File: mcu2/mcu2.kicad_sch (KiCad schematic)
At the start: 30 parts, among them J1 KF128-5.08, J2 Conn_01x26, J3 Conn_01x02, J4 Conn_01x01, J5 Conn_01x01, J6 Conn_01x01, J7 Conn_01x02, J8 Conn_01x26, Q1 WSF3085, Q2 PL4009, Q3 PL4009, U1 rp2040_zero, U2 motor_driver

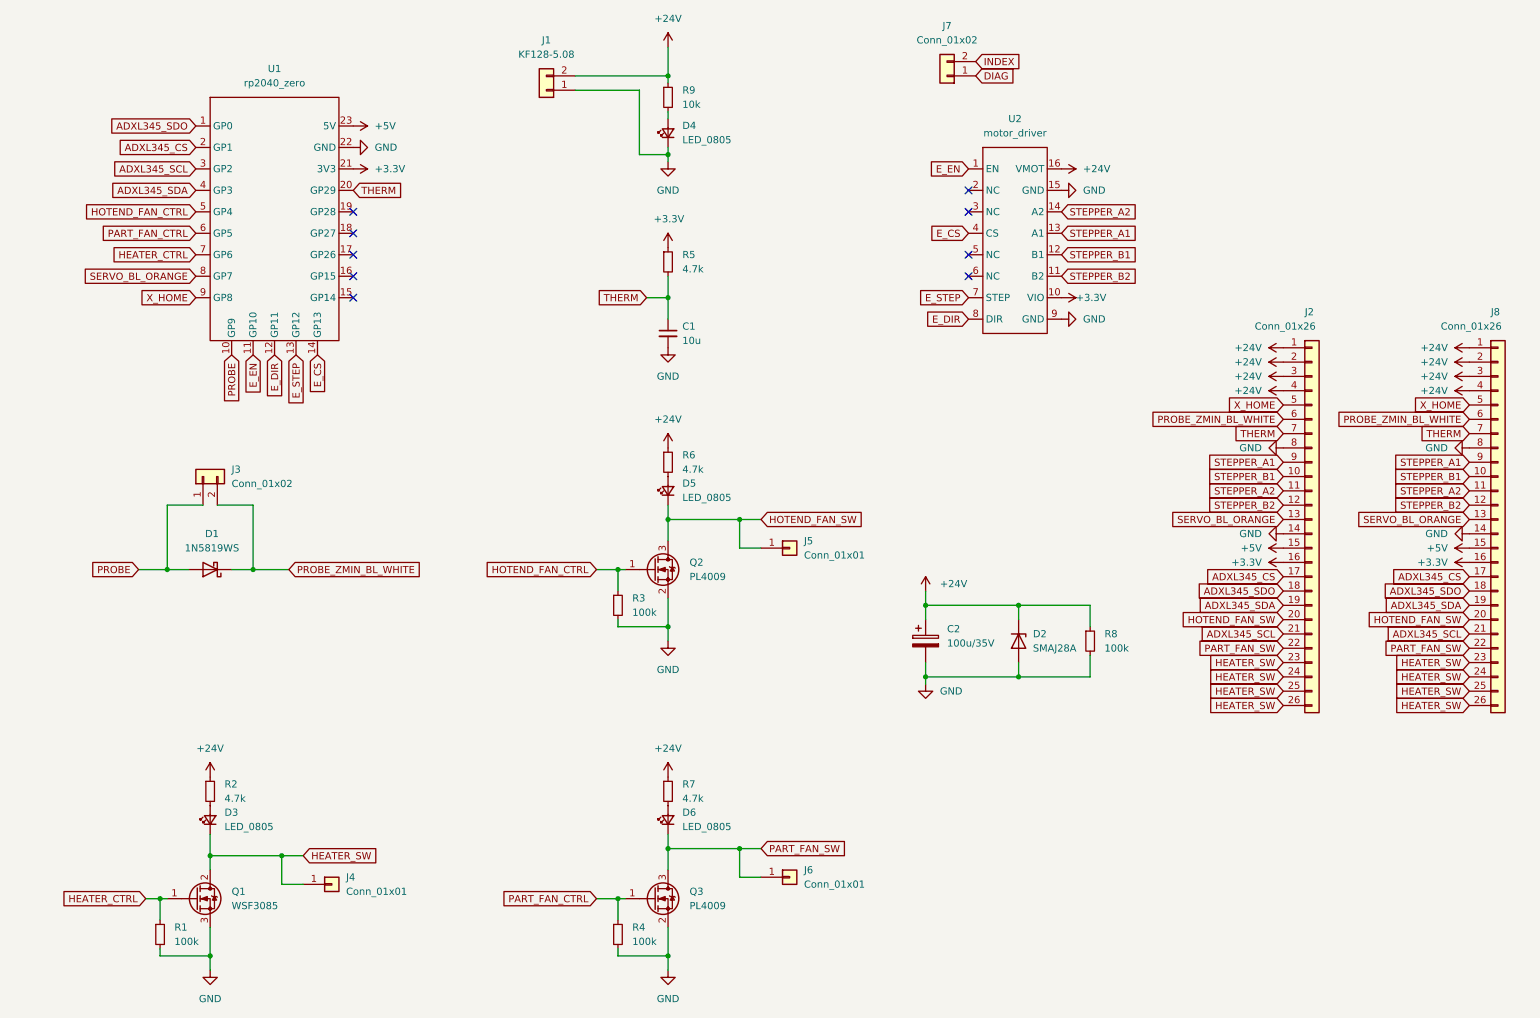
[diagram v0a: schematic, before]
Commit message: mcu schematic r3
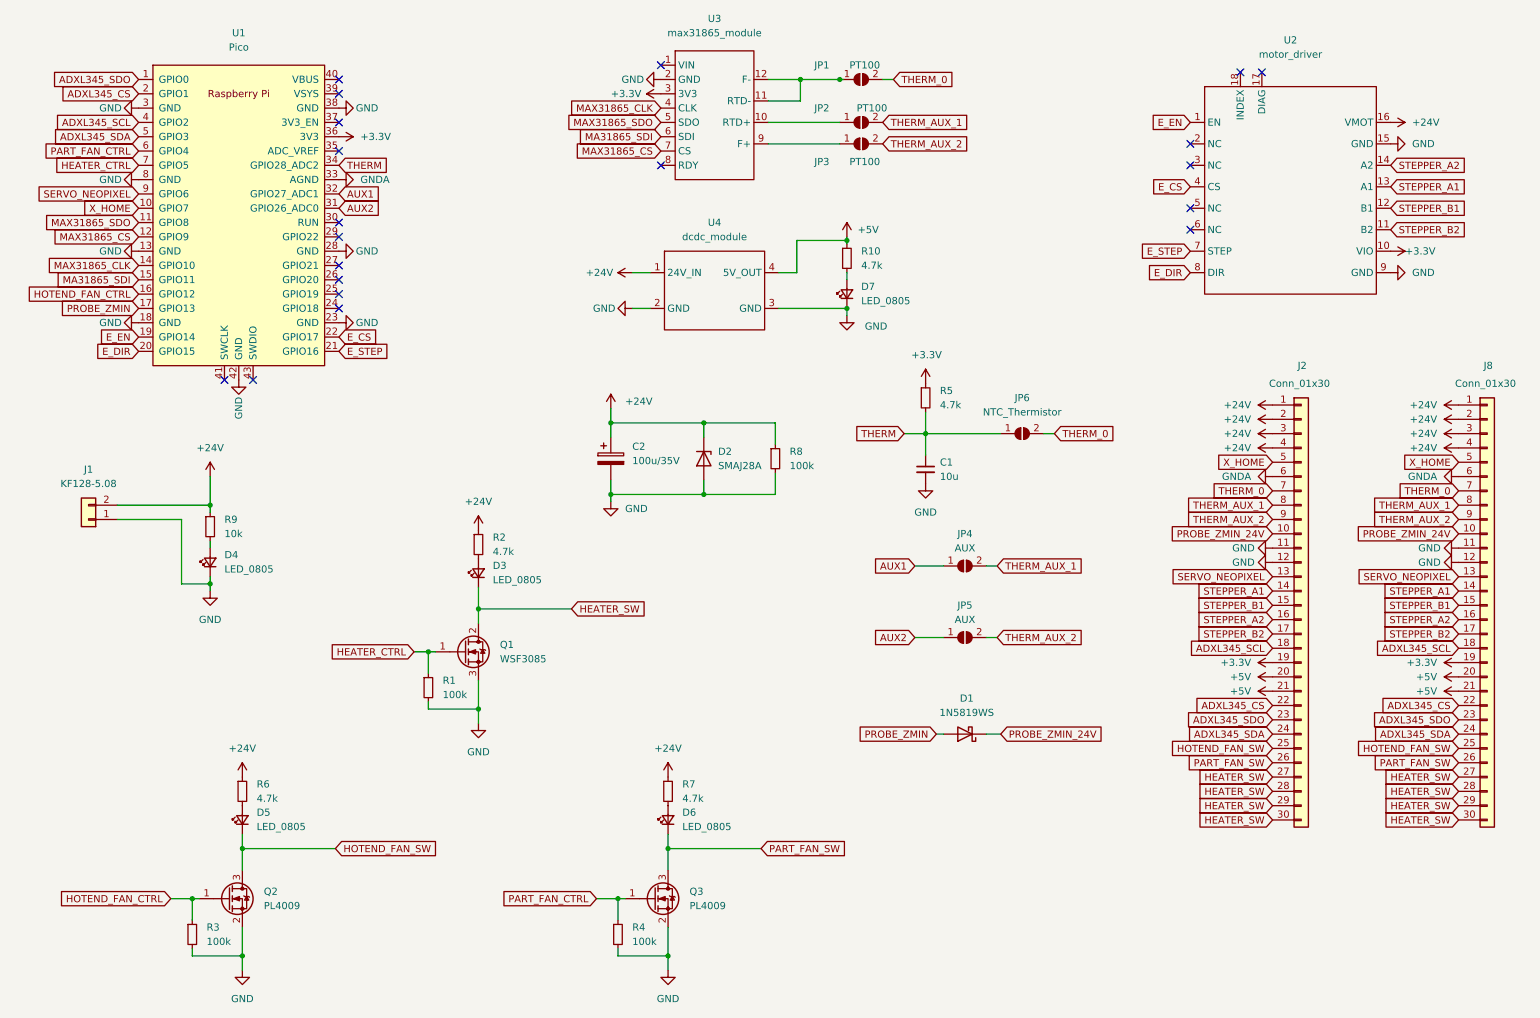
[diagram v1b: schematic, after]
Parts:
- removed J2, J8: Conn_01x26, FFCconnector:FFC26pinTH, symbol Connector_Generic:Conn_01x26
- removed J3, J7: Conn_01x02, Connector_PinHeader_2.54mm:PinHeader_1x02_P2.54mm_Vertical, symbol Connector_Generic:Conn_01x02
- removed J4, J5, J6: Conn_01x01, Connector_PinHeader_2.54mm:PinHeader_1x01_P2.54mm_Vertical, symbol Connector_Generic:Conn_01x01
- removed U1: rp2040_zero, rp2040_zero:RP2040Zero, symbol rp2040_zero:rp2040_zero
- removed U2: motor_driver, motor_driver:DIP-16_500, symbol motor_driver:motor_driver
- added D7: LED_0805, LED_SMD:LED_0805_2012Metric_Pad1.15x1.40mm_HandSolder, symbol Device:LED_Small
- added J2, J8: Conn_01x30, ffc_connectors:ffc-30pin, symbol Connector_Generic:Conn_01x30
- added JP1, JP2, JP3: PT100, symbol Jumper:SolderJumper_2_Open
- added JP4, JP5: AUX, symbol Jumper:SolderJumper_2_Open
- added JP6: NTC_Thermistor, symbol Jumper:SolderJumper_2_Open
- added R10: 4.7k, Resistor_SMD:R_0805_2012Metric_Pad1.20x1.40mm_HandSolder, symbol Device:R_Small
- added U1: Pico, RPi_Pico:RPi_Pico_SMD_TH, symbol RPi_Pico:Pico
- added U2: motor_driver, symbol ffc_mcu_library:motor_driver
- added U3: max31865_module, symbol ffc_mcu_library:max31865_module
- added U4: dcdc_module, symbol ffc_mcu_library:dcdc_module
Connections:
- net +24V: now also J2.1 (Pin_1), J2.2 (Pin_2), J2.3 (Pin_3), J2.4 (Pin_4), J8.1 (Pin_1), J8.2 (Pin_2), J8.3 (Pin_3), J8.4 (Pin_4), U2.16 (VMOT), U4.1 (24V_IN)
- net +3V3: now also J2.19 (Pin_19), J8.19 (Pin_19), U1.36 (3V3), U2.10 (VIO), U3.3 (3V3)
- net +5V: now also J2.20 (Pin_20), J2.21 (Pin_21), J8.20 (Pin_20), J8.21 (Pin_21), R10.1, U4.4 (5V_OUT)
- net ADXL345_CS: now also J2.22 (Pin_22), J8.22 (Pin_22), U1.2 (GPIO1)
- net ADXL345_SCL: now also J2.18 (Pin_18), J8.18 (Pin_18), U1.4 (GPIO2)
- net ADXL345_SDA: now also J2.24 (Pin_24), J8.24 (Pin_24), U1.5 (GPIO3)
- net ADXL345_SDO: now also J2.23 (Pin_23), J8.23 (Pin_23), U1.1 (GPIO0)
- net E_CS: now also U1.22 (GPIO17), U2.4 (CS)
- net E_DIR: now also U1.20 (GPIO15), U2.8 (DIR)
- net E_EN: now also U1.19 (GPIO14), U2.1 (EN)
- net E_STEP: now also U1.21 (GPIO16), U2.7 (STEP)
- net GND: now also D7.1 (K), J2.11 (Pin_11), J2.12 (Pin_12), J8.11 (Pin_11), J8.12 (Pin_12), U1.13 (GND), U1.18 (GND), U1.23 (GND), U1.28 (GND), U1.3 (GND), U1.38 (GND), U1.42 (GND), U1.8 (GND), U2.15 (GND), U2.9 (GND), U3.2 (GND), U4.2 (GND), U4.3 (GND)
- net HEATER_CTRL: now also U1.7 (GPIO5)
- net HEATER_SW: now also J2.27 (Pin_27), J2.28 (Pin_28), J2.29 (Pin_29), J2.30 (Pin_30), J8.27 (Pin_27), J8.28 (Pin_28), J8.29 (Pin_29), J8.30 (Pin_30)
- net HOTEND_FAN_CTRL: now also U1.16 (GPIO12)
- net HOTEND_FAN_SW: now also J2.25 (Pin_25), J8.25 (Pin_25)
- net PART_FAN_CTRL: now also U1.6 (GPIO4)
- net PART_FAN_SW: now also J2.26 (Pin_26), J8.26 (Pin_26)
- net STEPPER_A1: now also J2.14 (Pin_14), J8.14 (Pin_14), U2.13 (A1)
- net STEPPER_A2: now also J2.16 (Pin_16), J8.16 (Pin_16), U2.14 (A2)
- net STEPPER_B1: now also J2.15 (Pin_15), J8.15 (Pin_15), U2.12 (B1)
- net STEPPER_B2: now also J2.17 (Pin_17), J8.17 (Pin_17), U2.11 (B2)
- net THERM: now also JP6.1 (A), U1.34 (GPIO28_ADC2)
- net X_HOME: now also J2.5 (Pin_5), J8.5 (Pin_5), U1.10 (GPIO7)
- net PROBE renamed PROBE_ZMIN
- net PROBE_ZMIN: now also U1.17 (GPIO13)
- net PROBE_ZMIN_BL_WHITE renamed PROBE_ZMIN_24V
- net PROBE_ZMIN_24V: now also J2.10 (Pin_10), J8.10 (Pin_10)
- new net: JP2.1 (A), U3.10 (RTD+)
- new net: JP1.1 (A), U3.11 (RTD-), U3.12 (F-)
- new net: JP3.1 (A), U3.9 (F+)
- new net: D7.2 (A), R10.2
- new net AUX1: JP4.1 (A), U1.32 (GPIO27_ADC1)
- new net AUX2: JP5.1 (A), U1.31 (GPIO26_ADC0)
- new net GNDA: J2.6 (Pin_6), J8.6 (Pin_6), U1.33 (AGND)
- new net MA31865_SDI: U1.15 (GPIO11), U3.6 (SDI)
- new net MAX31865_CLK: U1.14 (GPIO10), U3.4 (CLK)
- new net MAX31865_CS: U1.12 (GPIO9), U3.7 (CS)
- new net MAX31865_SDO: U1.11 (GPIO8), U3.5 (SDO)
- new net SERVO_NEOPIXEL: J2.13 (Pin_13), J8.13 (Pin_13), U1.9 (GPIO6)
- new net THERM_0: J2.7 (Pin_7), J8.7 (Pin_7), JP1.2 (B), JP6.2 (B)
- new net THERM_AUX_1: J2.8 (Pin_8), J8.8 (Pin_8), JP2.2 (B), JP4.2 (B)
- new net THERM_AUX_2: J2.9 (Pin_9), J8.9 (Pin_9), JP3.2 (B), JP5.2 (B)
- no-connect marks 9 -> 20
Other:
- moved on the sheet: C1, C2, D1, D2, D3, D4, D5, J1, Q1, Q2, R1, R2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

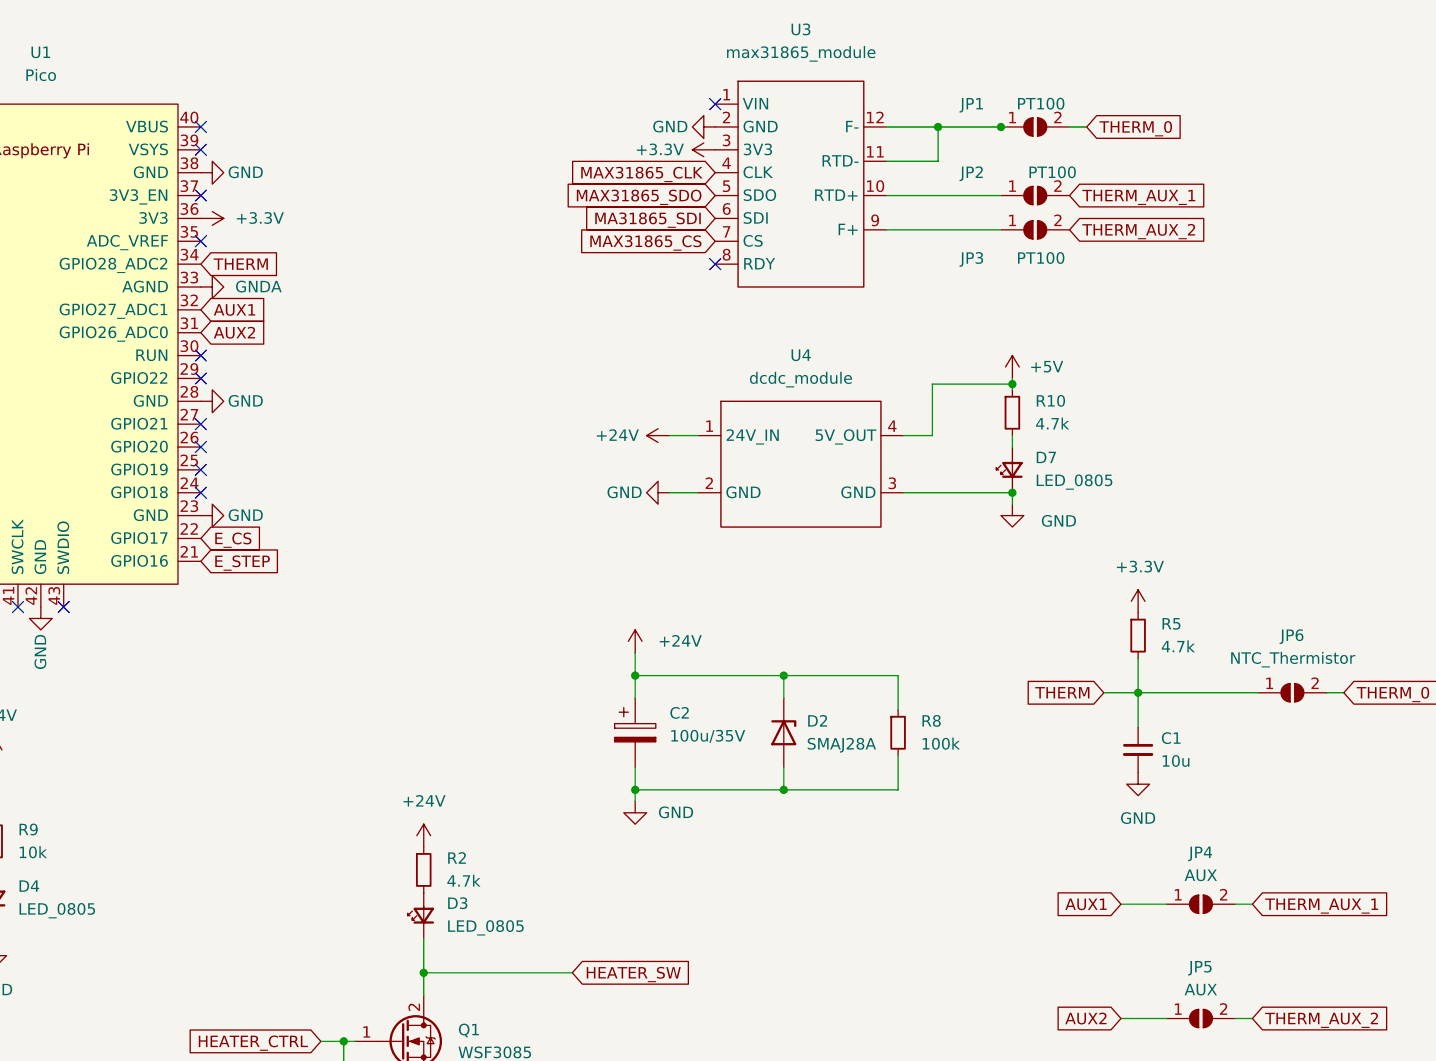
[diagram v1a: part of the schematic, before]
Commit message: add footprints
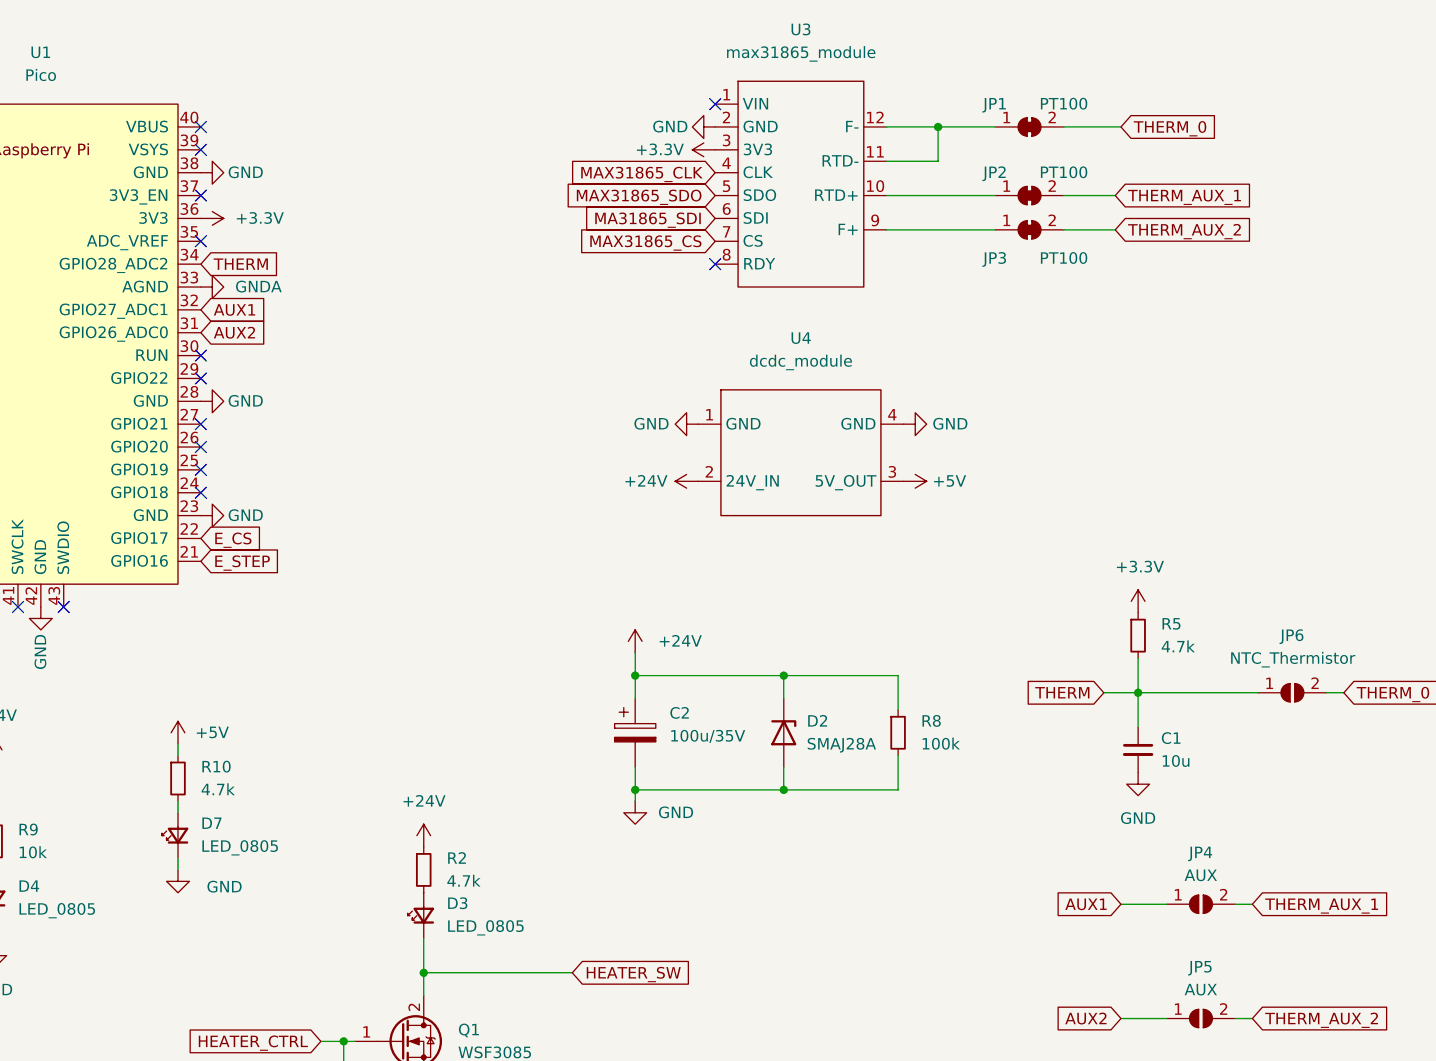
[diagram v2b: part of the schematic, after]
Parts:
- removed JP1, JP2, JP3: PT100, symbol Jumper:SolderJumper_2_Open
- added JP1, JP2, JP3: PT100, Jumper:SolderJumper-2_P1.3mm_Bridged_RoundedPad1.0x1.5mm, symbol Jumper:SolderJumper_2_Bridged
- JP4, JP5, JP6: footprint (none) -> Jumper:SolderJumper-2_P1.3mm_Open_RoundedPad1.0x1.5mm
- U2: footprint (none) -> ffc_connectors:motor_driver
- U3: footprint (none) -> ffc_connectors:adafruit_max31865_module
- U4: footprint (none) -> ffc_connectors:dcdc_24v_5v_module
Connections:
- net +24V: now also U4.2 (24V_IN); no longer U4.1 (24V_IN)
- net +5V: now also U4.3 (5V_OUT); no longer U4.4 (5V_OUT)
- net GND: now also U4.1 (GND), U4.4 (GND); no longer U4.2 (GND), U4.3 (GND)
- net THERM_0: now also JP1.2 (B)
- net THERM_AUX_1: now also JP2.2 (B)
- net THERM_AUX_2: now also JP3.2 (B)
- net at U3.10 (RTD+): now also JP2.1 (A)
- net at U3.11 (RTD-), U3.12 (F-): now also JP1.1 (A)
- net at U3.9 (F+): now also JP3.1 (A)
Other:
- moved on the sheet: D7, R10
